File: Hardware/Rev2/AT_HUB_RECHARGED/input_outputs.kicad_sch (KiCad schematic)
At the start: 25 parts, among them J10 IN3, J11 IN4, J12 IN5, J3 OUT1, J4 OUT2, J5 OUT3, J6 OUT4, J7 OUT5, J8 IN1, J9 IN2, U2 TLP241A(TP1,F, U3 TLP241A(TP1,F, U4 TLP241A(TP1,F, U5 TLP241A(TP1,F, U6 TLP241A(TP1,F

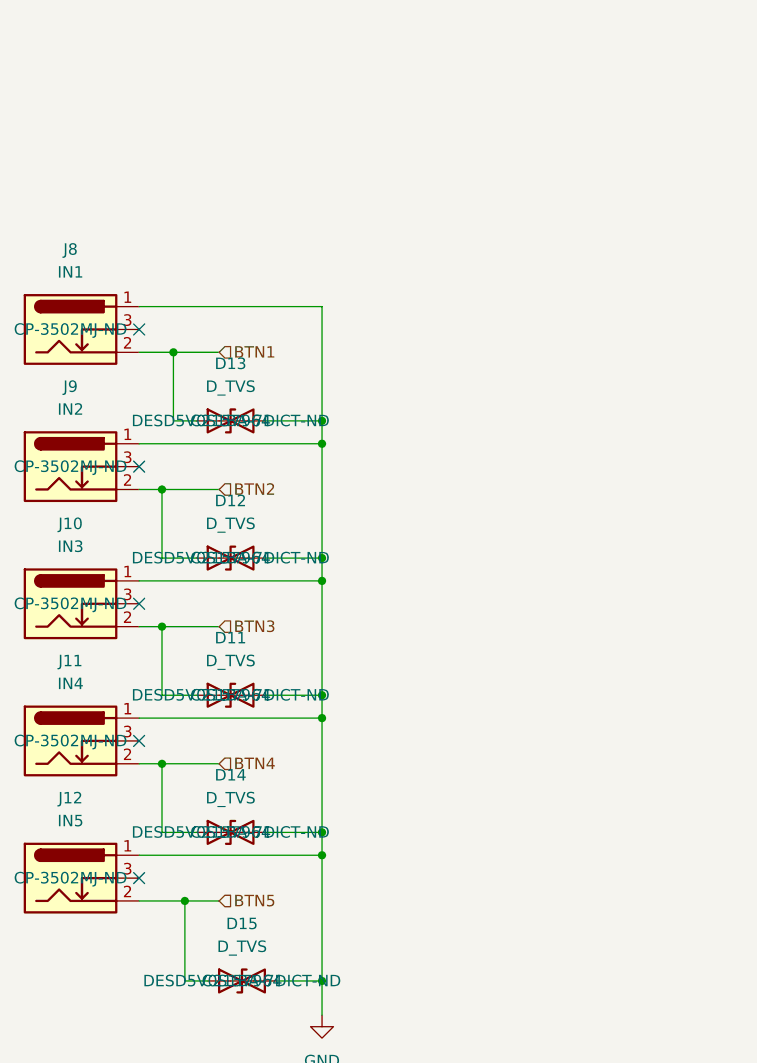
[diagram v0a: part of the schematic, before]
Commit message: Done the design will verify
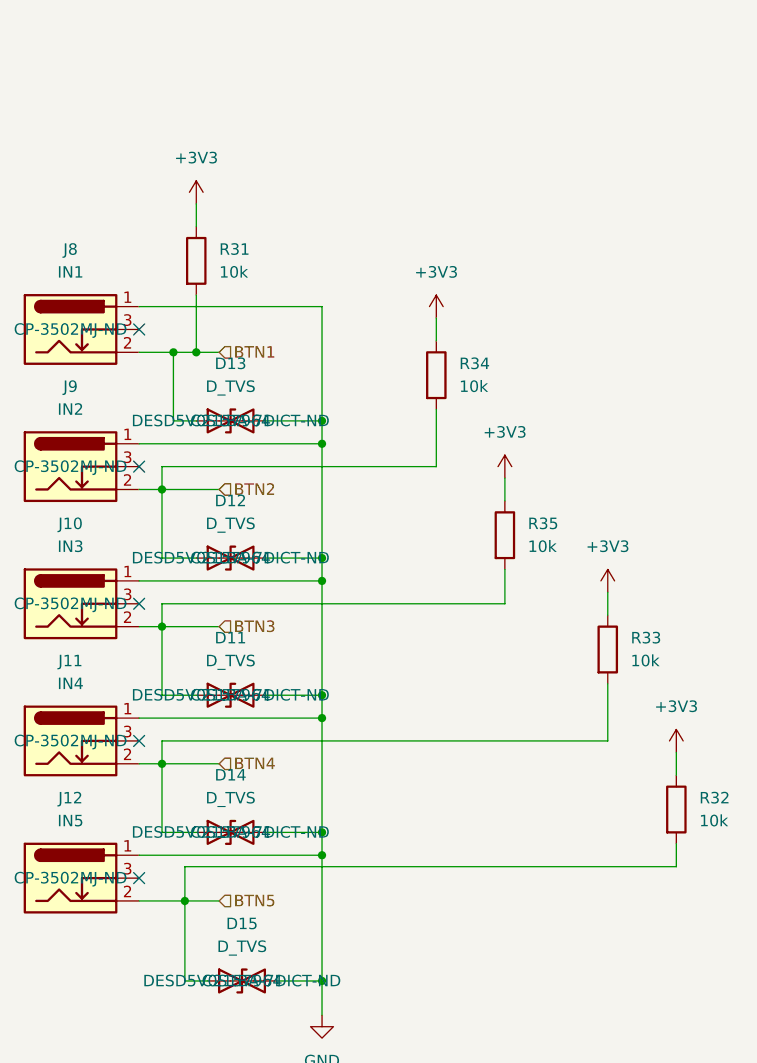
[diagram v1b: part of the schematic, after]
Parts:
- added R31, R32, R33, R34, R35: 10k, Resistor_SMD:R_0402_1005Metric, symbol Device:R
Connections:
- net BTN1: now also R31.2
- net BTN2: now also R34.2
- net BTN3: now also R35.2
- net BTN4: now also R33.2
- net BTN5: now also R32.2
- new net +3V3: R31.1, R32.1, R33.1, R34.1, R35.1
